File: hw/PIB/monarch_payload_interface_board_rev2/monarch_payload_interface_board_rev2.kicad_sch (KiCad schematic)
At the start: 0 parts

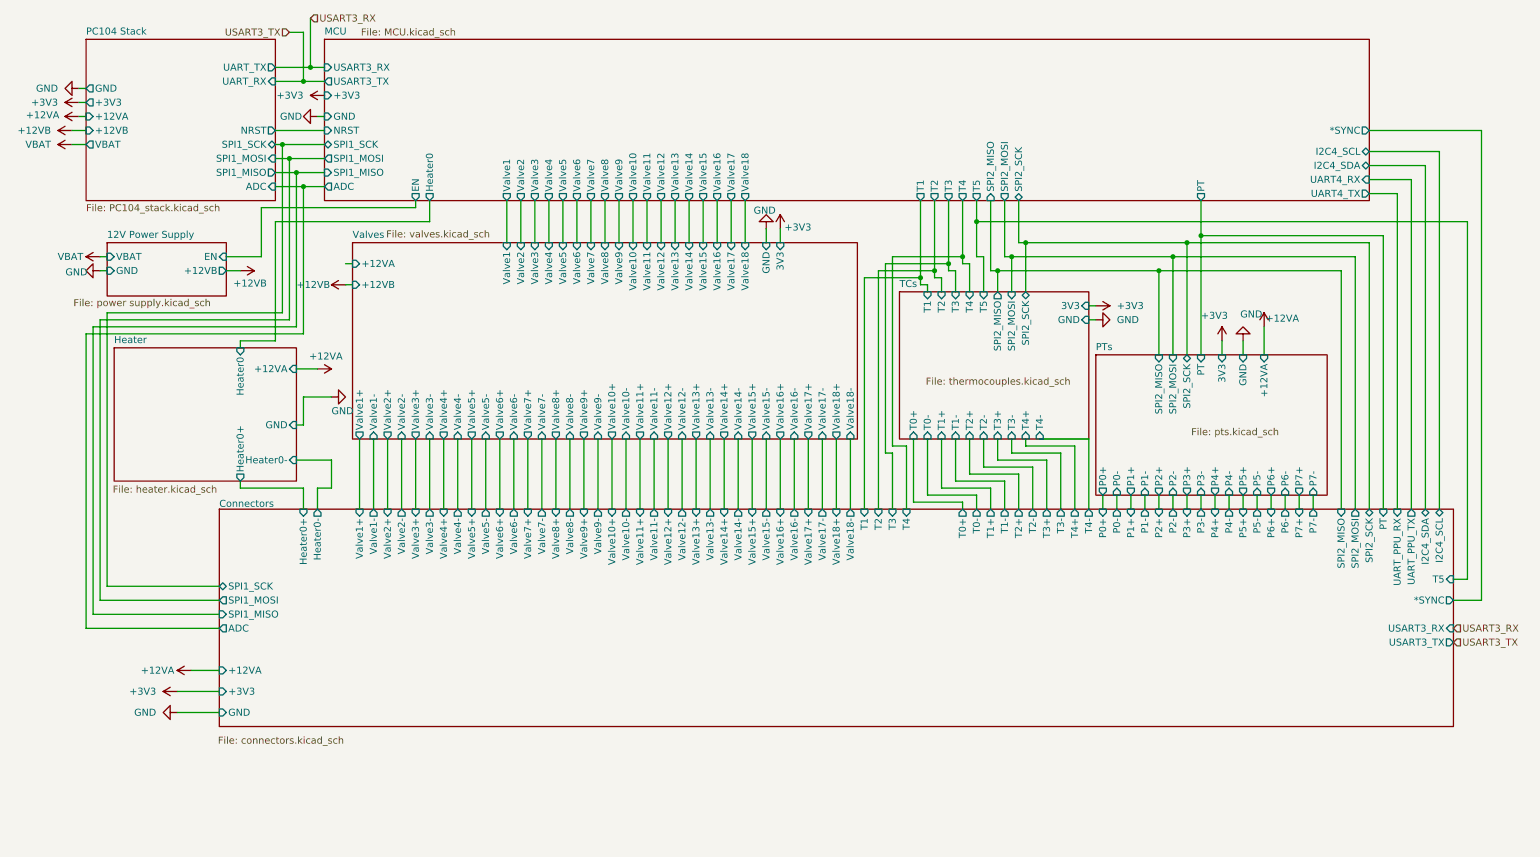
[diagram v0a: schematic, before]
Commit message: Layout Rev Done - NO DRC Check
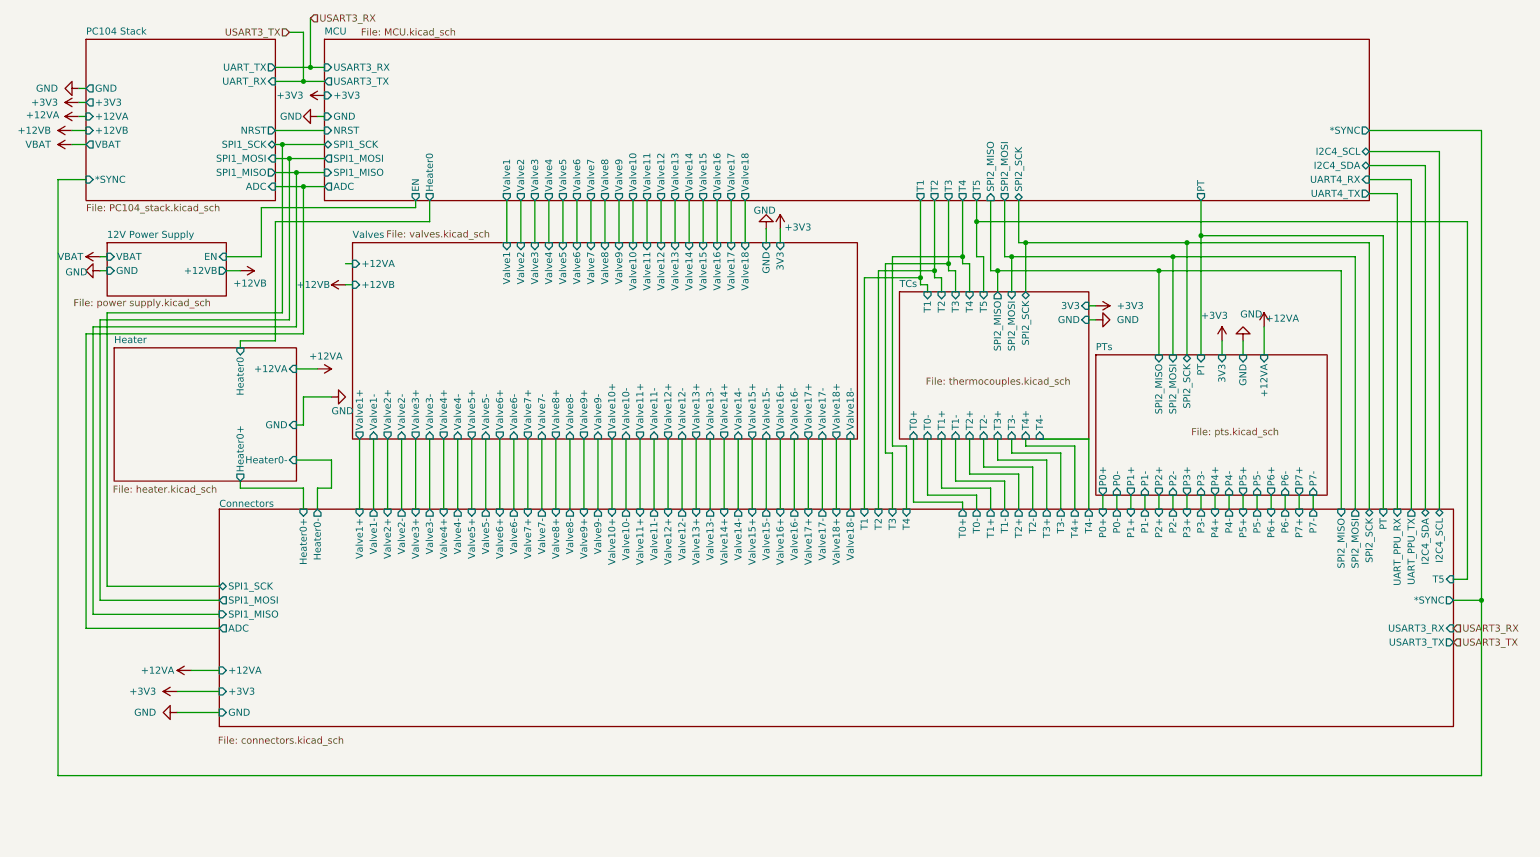
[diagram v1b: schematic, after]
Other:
- sheet PC104 Stack ports: added *SYNC; removed none
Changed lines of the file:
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@@
 	)
 	(junction
+		(at 278.13 119.38)
+		(diameter 0)
+		(color 0 0 0 0)
+	)
+	(junction
 		(at 190.5 59.69)
 		(diameter 0)
@@
 	(wire
 		(pts
+			(xy 20.32 151.13) (xy 278.13 151.13)
+		)
+		(stroke
+			(width 0)
+			(type default)
+		)
+	)
+	(wire
+		(pts
 			(xy 242.57 100.33) (xy 242.57 102.87)
 		)
@@
 	(wire
 		(pts
+			(xy 278.13 151.13) (xy 278.13 119.38)
+		)
+		(stroke
+			(width 0)
+			(type default)
+		)
+	)
+	(wire
+		(pts
 			(xy 59.69 34.29) (xy 68.58 34.29)
 		)
@@
 	(wire
 		(pts
+			(xy 25.4 43.18) (xy 20.32 43.18)
+		)
+		(stroke
+			(width 0)
+			(type default)
+		)
+	)
+	(wire
+		(pts
 			(xy 63.5 87.63) (xy 64.77 87.63)
 		)
@@
 	(wire
 		(pts
+			(xy 20.32 43.18) (xy 20.32 151.13)
+		)
+		(stroke
+			(width 0)
+			(type default)
+		)
+	)
+	(wire
+		(pts
 			(xy 194.31 96.52) (xy 194.31 102.87)
 		)
@@
 			)
 		)
+		(pin "*SYNC" input
+			(at 25.4 43.18 180)
+			(effects
+				(font
+					(size 1.27 1.27)
+				)
+				(justify left)
+			)
+		)

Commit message: FINAL REVIEW DONE + A lot of fixes. DRC PASSED
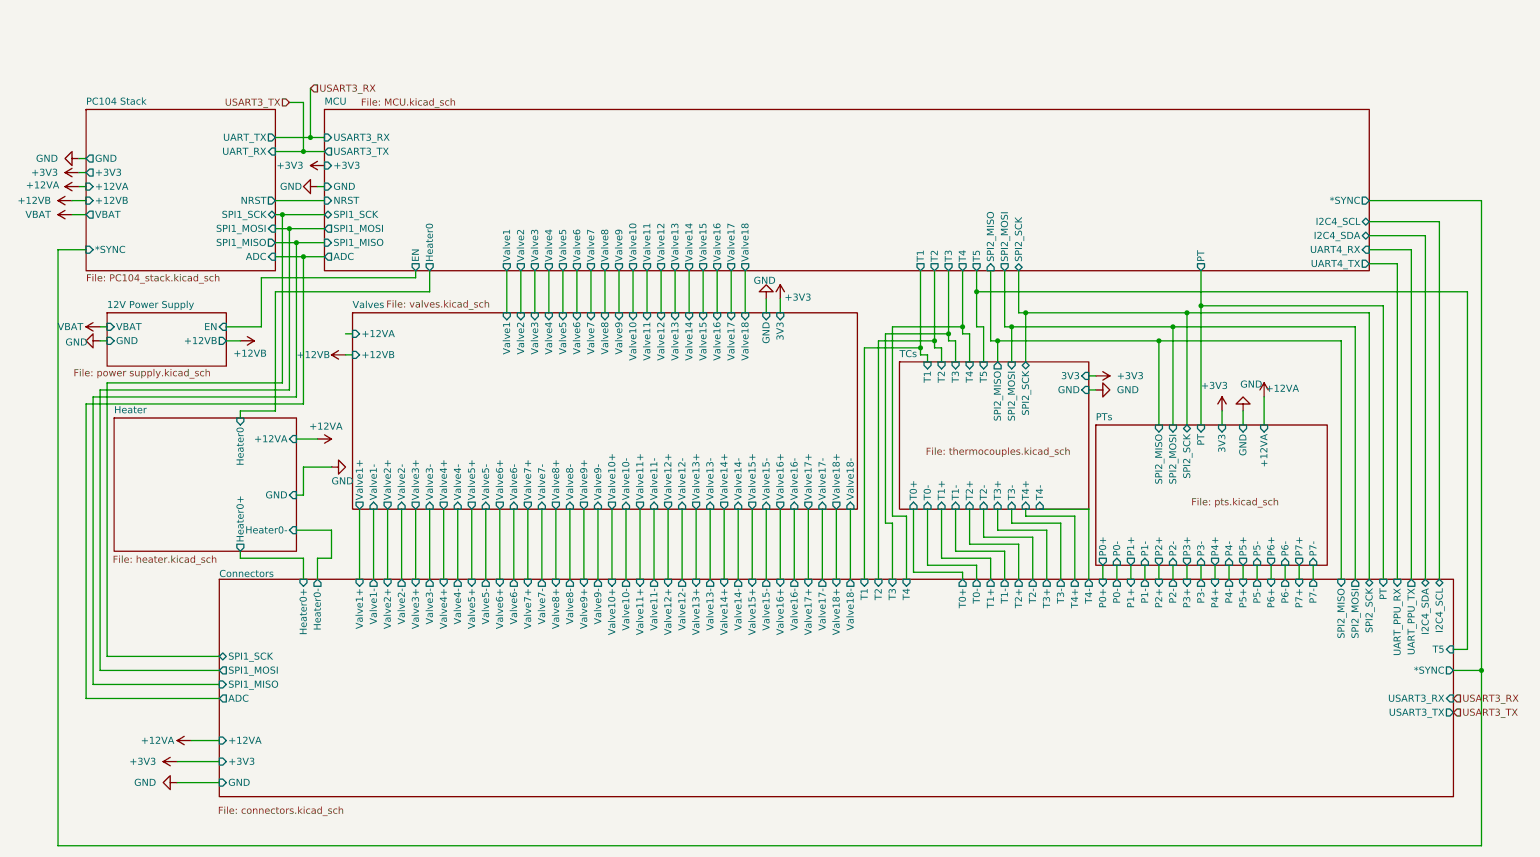
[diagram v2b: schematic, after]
